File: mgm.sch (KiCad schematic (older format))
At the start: 25 parts, among them M1 Fan_4pin, M2 Fan_4pin, T2 QT24A01, U1 rpi_cm4, U3 EMC2301, U4 rpi_cm4

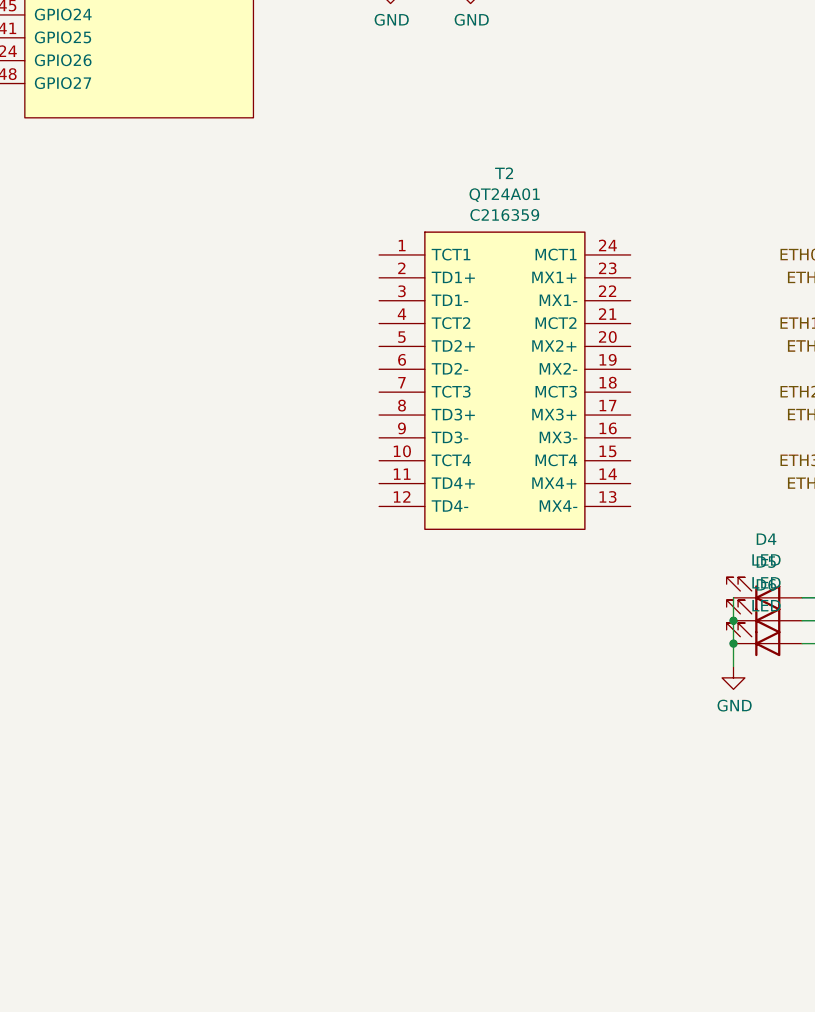
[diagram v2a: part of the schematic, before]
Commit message: use a 2x2 and a magjack
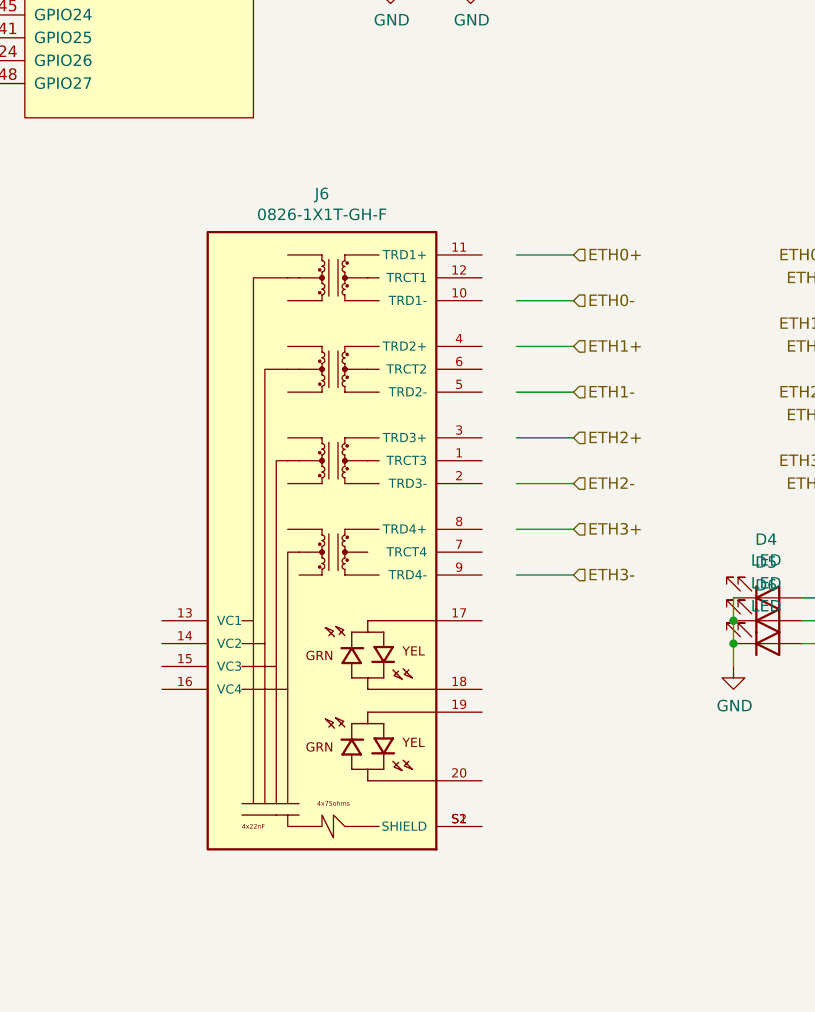
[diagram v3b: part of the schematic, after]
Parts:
- removed T2: QT24A01, dg_transformers:SOP100P1000X450-24N, symbol dg_transformers:QT24A01
- added J6: 0826-1X1T-GH-F, dg_connectors:BEL_0826-1X1T-GH-F, symbol dg_connectors:0826-1X1T-GH-F
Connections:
- wire segments 151 -> 159
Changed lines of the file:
@@
-$EndComp
-$Comp
-L dg_transformers:QT24A01 T?
-U 1 1 618693F9
-P 6550 3900
-AR Path="/620E19B3/618693F9" Ref="T?"  Part="1"
-AR Path="/613B6EFF/618693F9" Ref="T?"  Part="1"
-AR Path="/62156471/618693F9" Ref="T?"  Part="1"
-AR Path="/62171C6A/618693F9" Ref="T?"  Part="1"
-AR Path="/6218DDB9/618693F9" Ref="T?"  Part="1"
-AR Path="/613B5606/618693F9" Ref="T2"  Part="1"
-F 0 "T2" H 7100 4255 50  0000 C CNN
-F 1 "QT24A01" H 7100 4164 50  0000 C CNN
-F 2 "dg_transformers:SOP100P1000X450-24N" H 6700 2550 50  0001 L CNN
-F 3 "https://datasheet.lcsc.com/szlcsc/TNK-QT24A01_C216359.pdf" H 7500 3900 50  0001 L CNN
-F 4 "10/100/1000Base-T Single Port Transformer Module" H 6700 2450 50  0001 L CNN "Description"
-F 5 "4.5" H 7500 2350 50  0001 L CNN "Height"
-F 6 "TNK" H 6700 2350 50  0001 L CNN "Manufacturer_Name"
-F 7 "QT24A01" H 6950 2350 50  0001 L CNN "Manufacturer_Part_Number"
-F 8 "C216359" H 7100 4073 50  0000 C CNN "LCSC#"
-	1    6550 3900
-	1    0    0    -1
 $EndComp
 $Comp
@@
 Text HLabel 4600 2650 0    50   Input ~ 0
 c1_boot
+$Comp
+L dg_connectors:0826-1X1T-GH-F J6
+U 1 1 612127DD
+P 6200 5200
+F 0 "J6" H 6100 6767 50  0000 C CNN
+F 1 "0826-1X1T-GH-F" H 6100 6676 50  0000 C CNN
+F 2 "dg_connectors:BEL_0826-1X1T-GH-F" H 5750 6950 50  0001 L BNN
+F 3 "" H 6250 7100 50  0001 L BNN
+	1    6200 5200
+	-1   0    0    -1
+$EndComp
+Wire Wire Line
+	7400 4300 7150 4300
+Wire Wire Line
+	7150 4100 7400 4100
+Wire Wire Line
+	7400 3900 7150 3900
+Text HLabel 7400 4300 2    50   Input ~ 0
+ETH1+
+Text HLabel 7400 4100 2    50   Input ~ 0
+ETH0-
+Text HLabel 7400 3900 2    50   Input ~ 0
+ETH0+
+Text HLabel 7400 4500 2    50   Input ~ 0
+ETH1-
+Text HLabel 7400 4700 2    50   Input ~ 0
+ETH2+
+Wire Wire Line
+	7150 4500 7400 4500
+Wire Wire Line
+	7400 4700 7150 4700
+Text HLabel 7400 4900 2    50   Input ~ 0
+ETH2-
+Text HLabel 7400 5100 2    50   Input ~ 0
+ETH3+
+Wire Wire Line
+	7150 4900 7400 4900
+Wire Wire Line
+	7400 5100 7150 5100
+Text HLabel 7400 5300 2    50   Input ~ 0
+ETH3-
+Wire Wire Line
+	7150 5300 7400 5300
 $EndSCHEMATC
